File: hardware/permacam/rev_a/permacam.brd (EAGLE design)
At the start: 27 x 60 mm, 90 parts, among them J1 TC2030-JLINK-NL, Q1 PMDXB950UPEL, Q3 PMDXB950UPEL, Q5 PMDXB950UPEL, Q6 PMDXB950UPEL, U1 AB1815-T3, U10 NRF52840, U2 BQ25505, U3 EKMB1101111, U4 HM01B0-ANA, U7 MAX17222, U8 MAX44009, X1 32MHz, X3 32.768kHz, X4 ABS07-32.768KHZ-7-T

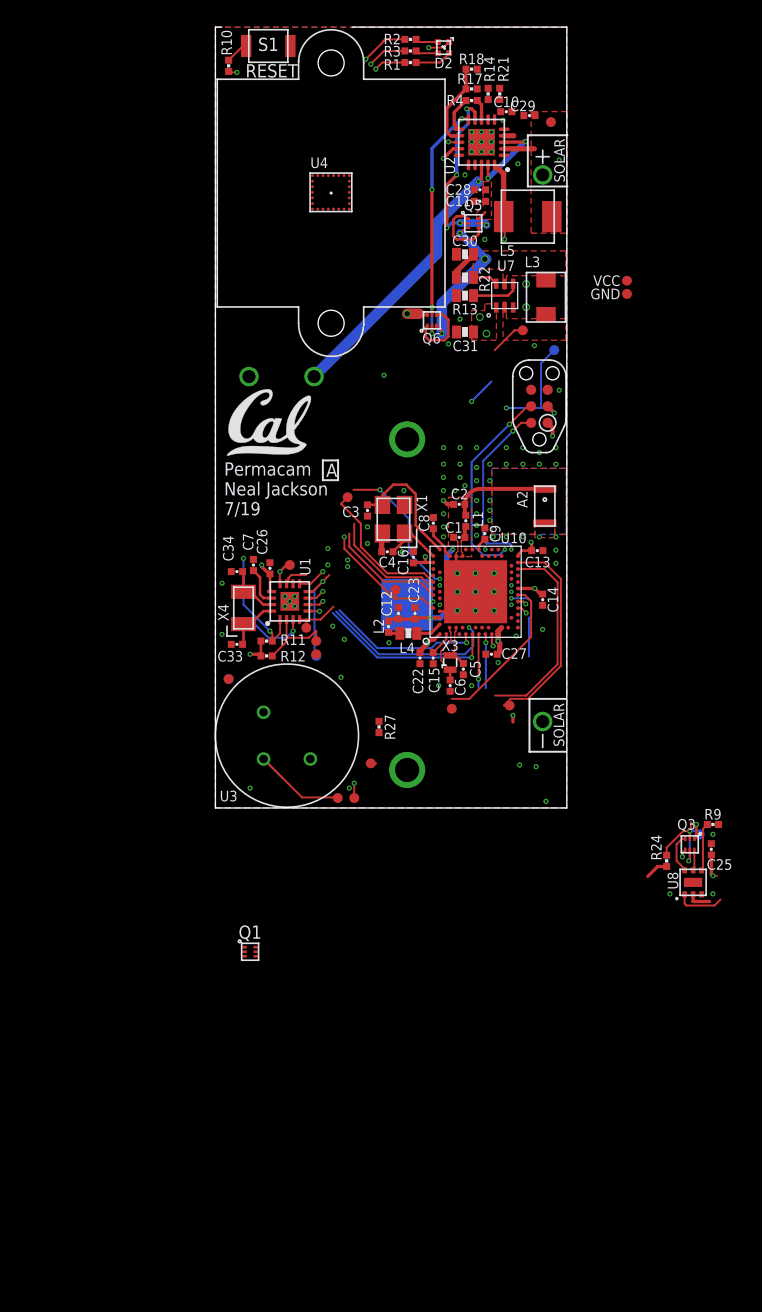
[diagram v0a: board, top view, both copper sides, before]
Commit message: clean and orient design blocks
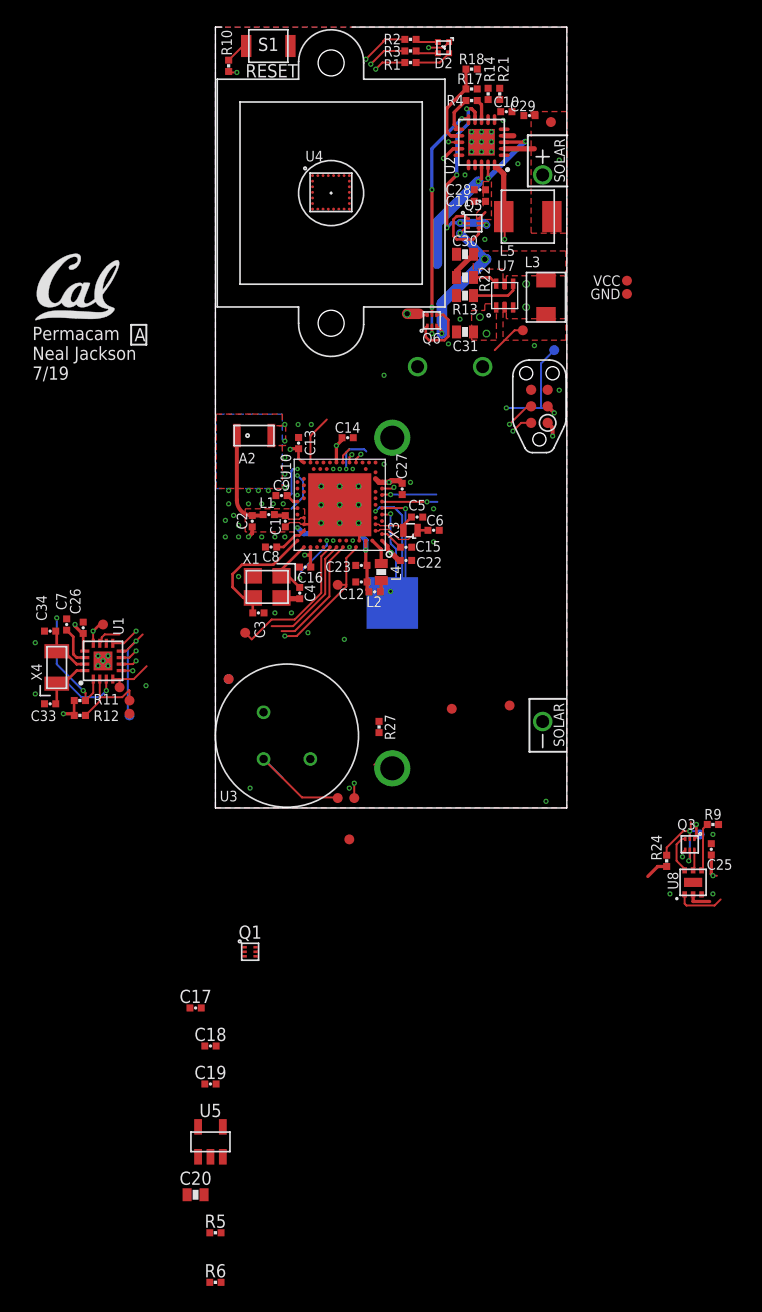
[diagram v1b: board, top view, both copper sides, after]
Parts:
- added C17, C18, C19: 0.1uF, passives:0402_CAP
- added C20: 10uF, passives:0603_CAP
- added R5, R6: 1k, passives:0402_RES
- added U5: MCP1810, chips:SOT-23-5
- moved A2 23.0 mm to (2.97, 28.6), turned to 0 degrees
- moved C13 20.1 mm to (6.39, 28.0), turned to 90 degrees
- moved C14 19.5 mm to (10.2, 28.4), turned to 0 degrees
- moved U$2 18.0 mm to (-13.8, 37.5)
- moved C2 16.0 mm to (2.83, 22.0), turned to 270 degrees
- moved C9 15.9 mm to (5.08, 24.0), turned to 180 degrees
- moved L1 15.1 mm to (4.10, 22.5), turned to 0 degrees
- moved C33 15.1 mm to (-12.7, 8.00)
- moved C34 15.1 mm to (-12.7, 13.6)
- moved C7 15.1 mm to (-11.4, 14.1)
- moved TP6 15.1 mm to (-8.64, 14.1)
- moved X4 15.1 mm to (-12.2, 10.8)
- moved C26 15.1 mm to (-10.2, 13.8)
- moved R11 15.1 mm to (-10.4, 8.26)
- moved R12 15.1 mm to (-10.4, 7.11)
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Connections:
- new net !CAM_EN: U5.2
- new net CAM_D0: U10.AD18, U4.17
- new net CAM_D1: U4.18
- new net CAM_D2: U4.19
- new net CAM_D3: U4.20
- new net CAM_INT: U10.V23, U4.1
- new net CAM_SCL: U10.T2
- new net CAM_SDA: R5.2, R6.2, U10.M2, U4.2, U4.3
- new net CAM_TRIG: U10.W24, U4.6
- new net FVLD: U10.AD20, U4.5
- new net LVLD: U10.AC19, U4.4
- new net MCLK: U10.AD16, U4.15
- new net PCLKO: U10.AC17, U4.16
- new net VCC28: C17.1, C18.1, C19.1, C20.1, R5.1, R6.1, U4.12, U4.13, U4.14, U4.23, U4.8, U5.3
- net !LT_EN: now also U10.Y23; no longer U10.AD20
- net GND: now also C17.2, C18.2, C19.2, C20.2, U4.10, U4.11, U4.24, U4.7, U4.9, U5.5
- net VCC: now also U5.1
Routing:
- net !LT_EN: track 23.9 -> 8.31 mm
- net LBST: track 24.3 -> 9.85 mm, vias 3 -> 2
- net !LT_INT: track 20.3 -> 7.52 mm
- net VSEC: track 32.4 -> 19.8 mm
- net VBAT_OK: track 13.6 -> 1.05 mm
- net !RST: track 36.0 -> 25.1 mm
- net !PIR_EN: track 12.1 -> 1.32 mm
- net SWDCLK: track 15.7 -> 5.34 mm
- net SWDIO: track 13.6 -> 4.31 mm
- net RTC_CS: track 12.9 -> 5.12 mm, vias 3 -> 2
- net LED_GREEN: track 17.6 -> 12.7 mm
- net LED_BLUE: track 16.7 -> 12.1 mm
- net LED_RED: track 14.3 -> 10.2 mm
- net PIR_OUT: track 14.9 -> 12.0 mm
- net !RTC_IRQ2: track 12.9 -> 10.7 mm, vias 2 -> 1
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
